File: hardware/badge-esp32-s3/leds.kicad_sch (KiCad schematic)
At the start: 0 parts

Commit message: RGB
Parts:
- added LED1: XL-2012RGBC, lcsc-lib:LED-SMD_4P-L2.0-W1.3-BR, symbol lcsc-lib:XL-2012RGBC
- added R22: 180Ω, PCM_JLCPCB:R_0805, symbol PCM_JLCPCB-Resistors:0805,180Ω
- added R23, R24: 150Ω, PCM_JLCPCB:R_0805, symbol PCM_JLCPCB-Resistors:0805,150Ω
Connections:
- new net: LED1.1, R22.2
- new net: LED1.2, R23.2
- new net: LED1.4, R24.1
- new net Blue: R24.2
- new net Green: R23.1
- new net Red: R22.1
- new net VCC_5V: LED1.3

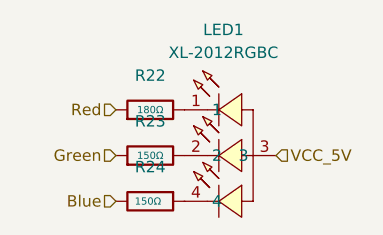
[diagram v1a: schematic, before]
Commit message: RGB
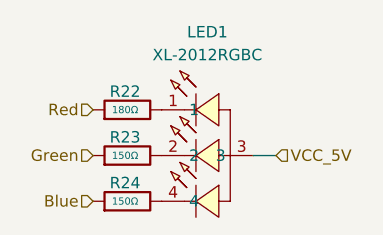
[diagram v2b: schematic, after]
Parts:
- removed R23, R24: 150Ω, PCM_JLCPCB:R_0805, symbol PCM_JLCPCB-Resistors:0805,150Ω
- added R23, R24: 150Ω, PCM_JLCPCB:R_0805, symbol PCM_JLCPCB-Resistors:0805,180Ω
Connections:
- net Blue: now also R24.1
- net Green: now also R23.1
- net at LED1.2: now also R23.2
- net at LED1.4: now also R24.2
